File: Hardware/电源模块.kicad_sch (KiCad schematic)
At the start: 34 parts, among them J4 Barrel_Jack_Switch_MountingPin, U2 EA3036C, U3 MP2225GJ

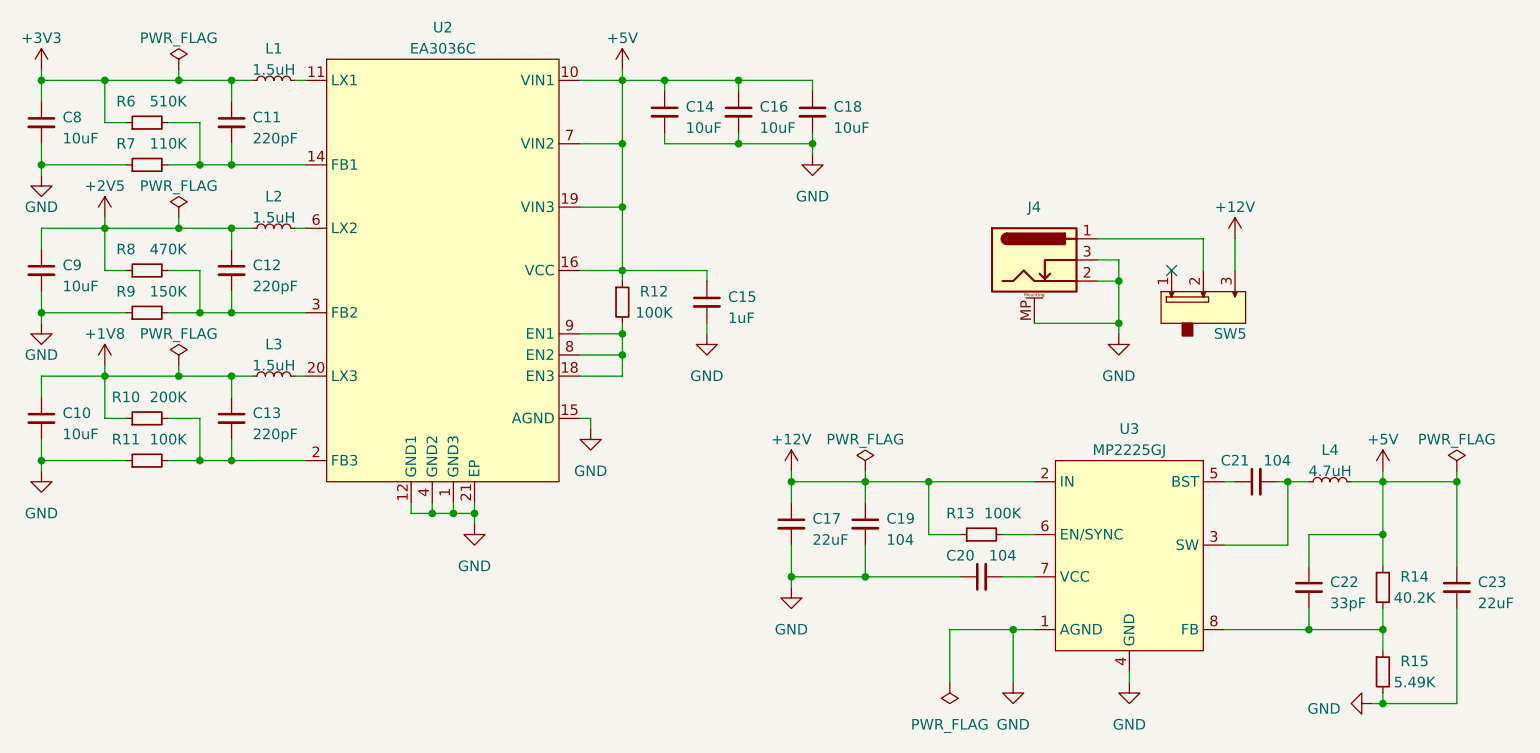
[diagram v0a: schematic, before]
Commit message: update
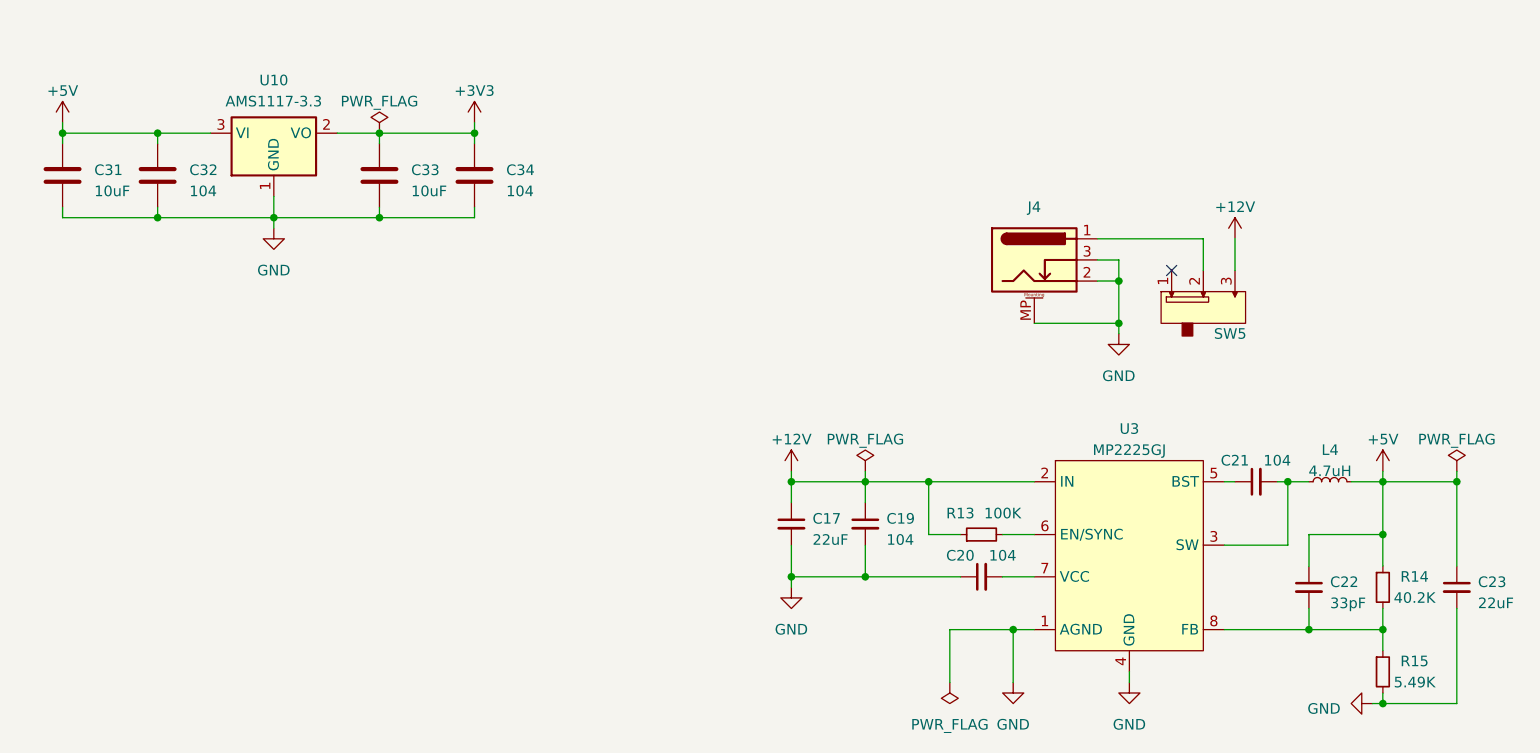
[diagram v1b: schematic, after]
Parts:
- removed C10, C14, C16, C18, C8, C9: 10uF, Capacitor_SMD:C_0402_1005Metric, symbol Device:C_Small
- removed C11, C12, C13: 220pF, Capacitor_SMD:C_0402_1005Metric, symbol Device:C_Small
- removed C15: 1uF, Capacitor_SMD:C_0402_1005Metric, symbol Device:C_Small
- removed L1, L2, L3: 1.5uH, Inductor_SMD:L_1206_3216Metric, symbol Device:L_Small
- removed R10: 200K, Resistor_SMD:R_0402_1005Metric, symbol Device:R_Small
- removed R11, R12: 100K, Resistor_SMD:R_0402_1005Metric, symbol Device:R_Small
- removed R6: 510K, Resistor_SMD:R_0402_1005Metric, symbol Device:R_Small
- removed R7: 110K, Resistor_SMD:R_0402_1005Metric, symbol Device:R_Small
- removed R8: 470K, Resistor_SMD:R_0402_1005Metric, symbol Device:R_Small
- removed R9: 150K, Resistor_SMD:R_0402_1005Metric, symbol Device:R_Small
- removed U2: EA3036C, Package_DFN_QFN:QFN-20-1EP_3x3mm_P0.4mm_EP1.65x1.65mm, symbol Power_Management:EA3036C
- added C31, C33: 10uF, Capacitor_SMD:C_0402_1005Metric, symbol Device:C
- added C32, C34: 104, Capacitor_SMD:C_0402_1005Metric, symbol Device:C
- added U10: AMS1117-3.3, Package_TO_SOT_SMD:SOT-223-3_TabPin2, symbol Regulator_Linear:AMS1117-3.3
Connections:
- net +3V3: now also C33.1, C34.1, U10.2 (VO)
- net +5V: now also C31.1, C32.1, U10.3 (VI)
- net GND: now also C31.2, C32.2, C33.2, C34.2, U10.1 (GND)
